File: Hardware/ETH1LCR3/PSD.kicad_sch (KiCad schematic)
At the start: 12 parts, among them U701 SN74LVC1G3157DB, U702 SN74LVC1G3157DB, U703 SN74LV1T34DBV, U704 SN74LV1T34DBV, U705 SN74LV1T34DBV, U706 TLV3501AIDBV

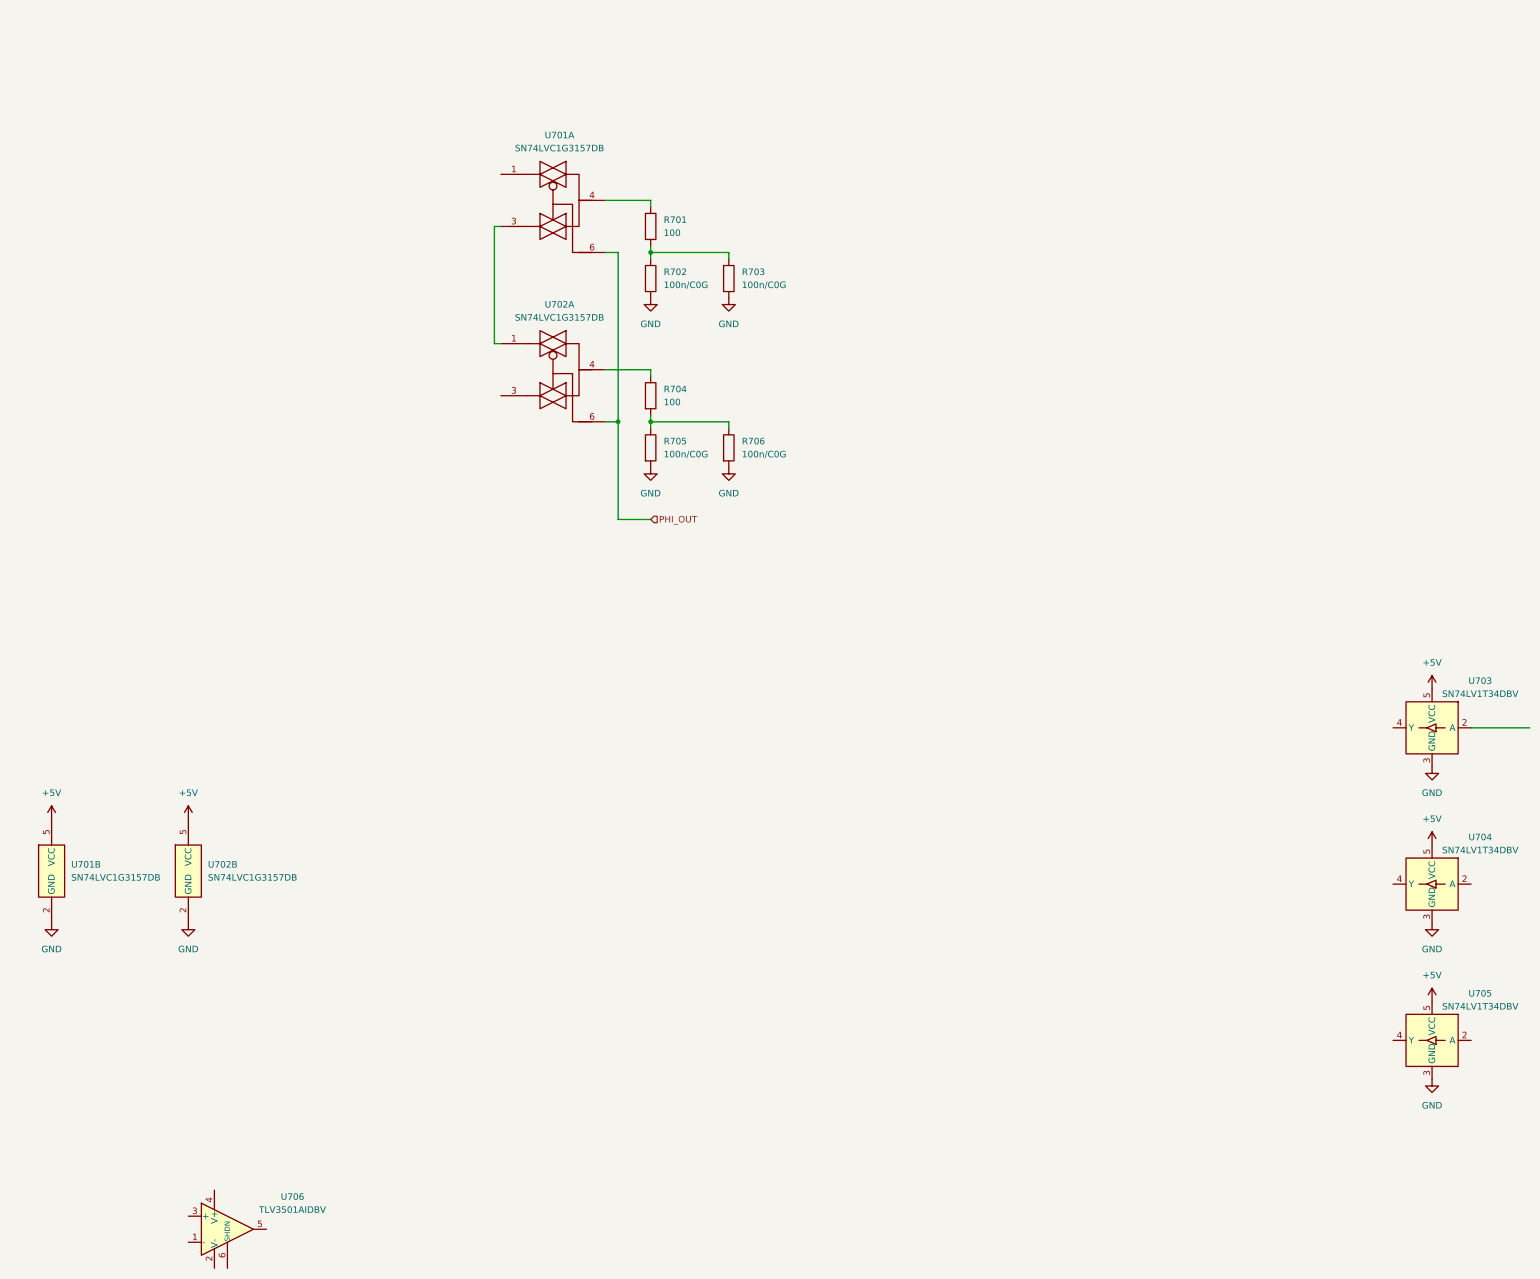
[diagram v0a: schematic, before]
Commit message: Hardware
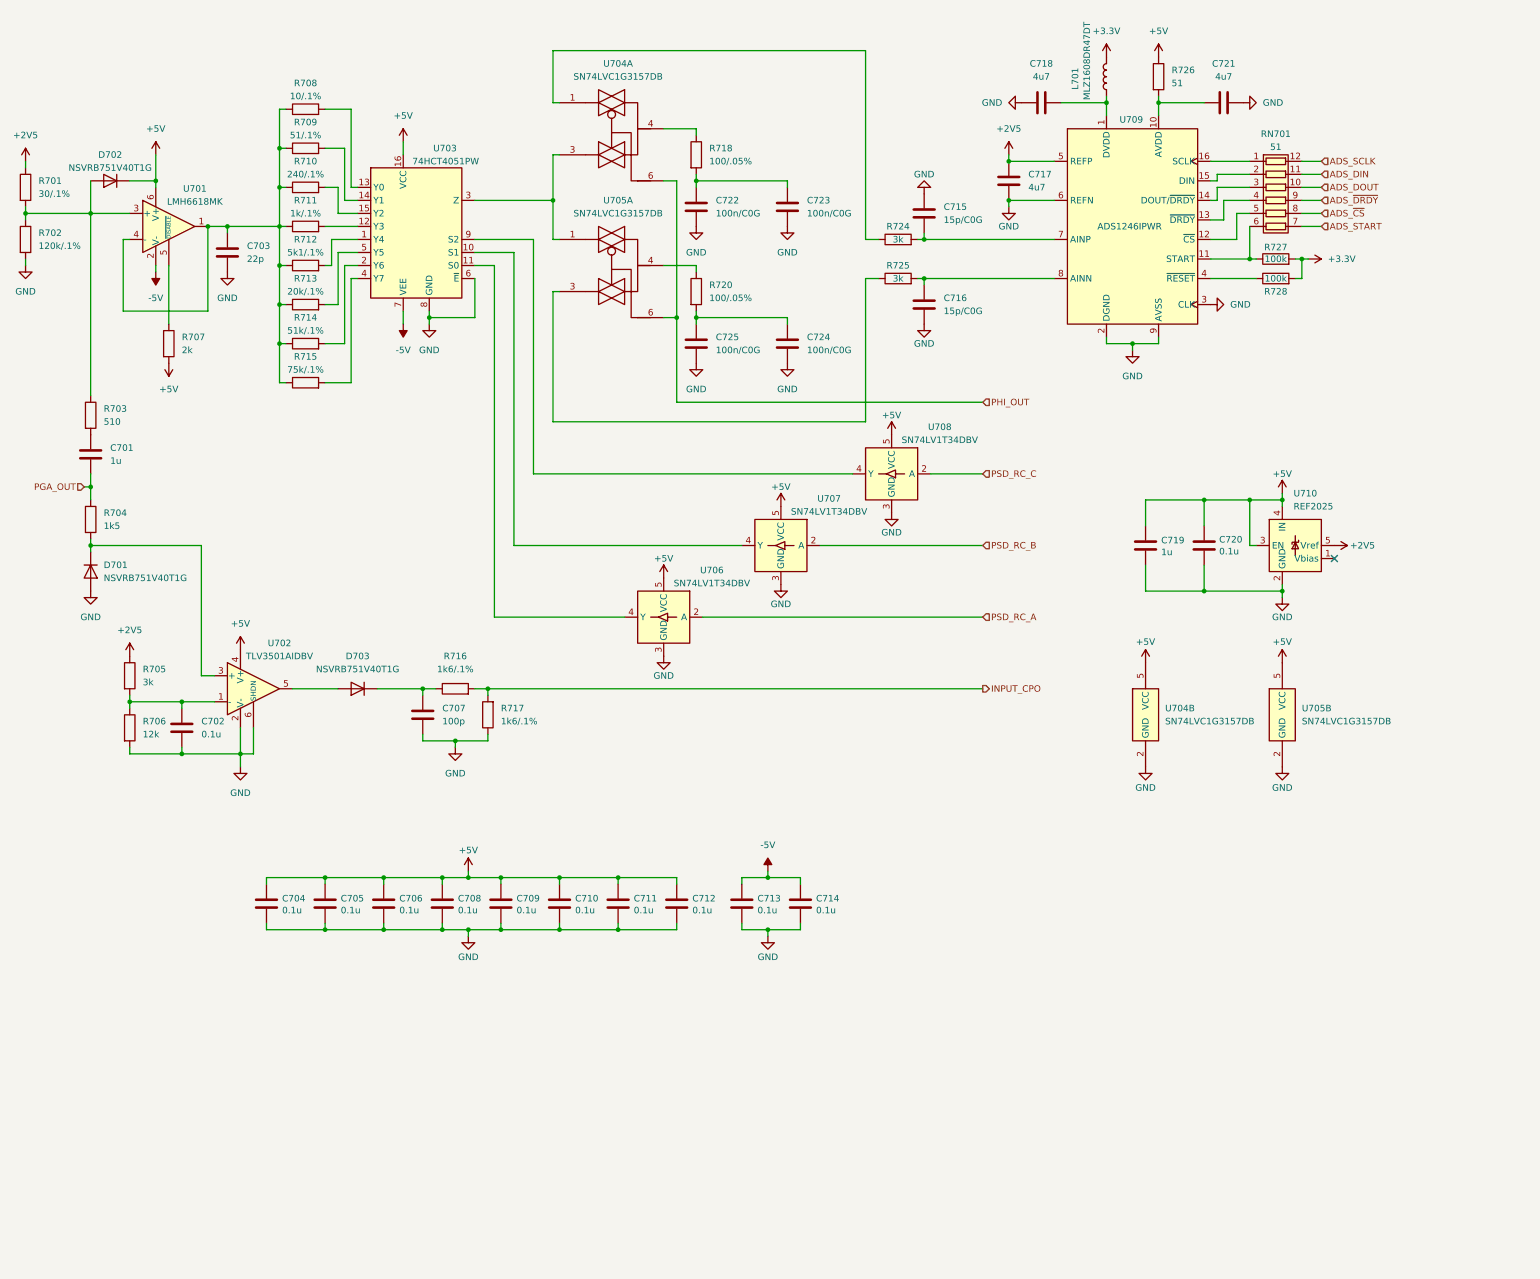
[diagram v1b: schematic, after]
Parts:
- added C701, C719: 1u, Capacitor_SMD:C_0603_1608Metric_Pad1.08x0.95mm_HandSolder, symbol Device:C
- added C702, C704, C705, C706, C708, C709, C710, C711, C712, C713, C714, C720: 0.1u, Capacitor_SMD:C_0603_1608Metric_Pad1.08x0.95mm_HandSolder, symbol Device:C
- added C703: 22p, Capacitor_SMD:C_0603_1608Metric_Pad1.08x0.95mm_HandSolder, symbol Device:C
- added C707: 100p, Capacitor_SMD:C_0603_1608Metric_Pad1.08x0.95mm_HandSolder, symbol Device:C
- added C715, C716: 15p/C0G, symbol Device:C
- added C717, C718, C721: 4u7, symbol Device:C
- added C722, C723, C724, C725: 100n/C0G, symbol Device:C
- added D701, D702, D703: NSVRB751V40T1G, symbol Device:D
- added L701: MLZ1608DR47DT, Inductor_SMD:L_0603_1608Metric_Pad1.05x0.95mm_HandSolder, symbol Device:L
- added R701: 30/.1%, Resistor_SMD:R_0603_1608Metric_Pad0.98x0.95mm_HandSolder, symbol Device:R
- added R704: 1k5, Resistor_SMD:R_0603_1608Metric_Pad0.98x0.95mm_HandSolder, symbol Device:R
- added R707: 2k, Resistor_SMD:R_0603_1608Metric_Pad0.98x0.95mm_HandSolder, symbol Device:R
- added R708: 10/.1%, Resistor_SMD:R_0603_1608Metric_Pad0.98x0.95mm_HandSolder, symbol Device:R
- added R709: 51/.1%, Resistor_SMD:R_0603_1608Metric_Pad0.98x0.95mm_HandSolder, symbol Device:R
- added R710: 240/.1%, Resistor_SMD:R_0603_1608Metric_Pad0.98x0.95mm_HandSolder, symbol Device:R
- added R711: 1k/.1%, Resistor_SMD:R_0603_1608Metric_Pad0.98x0.95mm_HandSolder, symbol Device:R
- added R712: 5k1/.1%, Resistor_SMD:R_0603_1608Metric_Pad0.98x0.95mm_HandSolder, symbol Device:R
- added R713: 20k/.1%, Resistor_SMD:R_0603_1608Metric_Pad0.98x0.95mm_HandSolder, symbol Device:R
- added R714: 51k/.1%, Resistor_SMD:R_0603_1608Metric_Pad0.98x0.95mm_HandSolder, symbol Device:R
- added R715: 75k/.1%, Resistor_SMD:R_0603_1608Metric_Pad0.98x0.95mm_HandSolder, symbol Device:R
- added R716, R717: 1k6/.1%, Resistor_SMD:R_0603_1608Metric_Pad0.98x0.95mm_HandSolder, symbol Device:R
- added R724, R725: 3k, Resistor_SMD:R_0603_1608Metric_Pad0.98x0.95mm_HandSolder, symbol Device:R
- added R726: 51, Resistor_SMD:R_0603_1608Metric_Pad0.98x0.95mm_HandSolder, symbol Device:R
- added R727, R728: 100k, Resistor_SMD:R_0603_1608Metric_Pad0.98x0.95mm_HandSolder, symbol Device:R
- added RN701: 51, symbol Device:R_Pack06
- added U701: LMH6618MK, Package_TO_SOT_SMD:TSOT-23-6_HandSoldering, symbol ETH1LCR3:LMH6618MK
- added U703: 74HCT4051PW, Package_SO:TSSOP-16_4.4x5mm_P0.65mm, symbol ETH1LCR3:74HCT4051PW
- added U709: ADS1246IPWR, Package_SO:TSSOP-16_4.4x5mm_P0.65mm, symbol ETH1LCR3:ADS1246IPWR
- added U710: REF2025, Package_TO_SOT_SMD:SOT-23-5, symbol Reference_Voltage:REF2025
- R702: value 100n/C0G -> 120k/.1%; footprint (none) -> Resistor_SMD:R_0603_1608Metric_Pad0.98x0.95mm_HandSolder
- R703: value 100n/C0G -> 510; footprint (none) -> Resistor_SMD:R_0603_1608Metric_Pad0.98x0.95mm_HandSolder
- R705: value 100n/C0G -> 3k; footprint (none) -> Resistor_SMD:R_0603_1608Metric_Pad0.98x0.95mm_HandSolder
- R706: value 100n/C0G -> 12k; footprint (none) -> Resistor_SMD:R_0603_1608Metric_Pad0.98x0.95mm_HandSolder
- R718: renamed from R701; value 100 -> 100/.05%; footprint (none) -> Resistor_SMD:R_0603_1608Metric_Pad0.98x0.95mm_HandSolder
- R720: renamed from R704; value 100 -> 100/.05%; footprint (none) -> Resistor_SMD:R_0603_1608Metric_Pad0.98x0.95mm_HandSolder
- U704: renamed from U701; footprint (none) -> Package_TO_SOT_SMD:SOT-23-6_Handsoldering
- U705: renamed from U702; footprint (none) -> Package_TO_SOT_SMD:SOT-23-6_Handsoldering
- renumbered U706 to U702, U705 to U706, U704 to U707, U703 to U708
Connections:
- net +5V: now also U702.4 (V+), C704.1, C705.1, C706.1, C708.1, C709.1, C710.1, C711.1, C712.1, C719.1, C720.1, D702.1 (K), R707.2, R726.1, U701.6 (V+), U703.16 (VCC), U710.3 (EN), U710.4 (IN)
- net GND: now also U702.2 (V-), U702.6 (SHDN), C702.2, C703.2, C704.2, C705.2, C706.2, C707.2, C708.2, C709.2, C710.2, C711.2, C712.2, C713.2, C714.2, C715.1, C716.2, C717.2, C718.1, C719.2, C720.2, C721.2, C722.2, C723.2, C724.2, C725.2, D701.2 (A), R717.1, U703.6 (~{E}), U703.8 (GND), U709.2 (DGND), U709.3 (CLK), U709.6 (REFN), U709.9 (AVSS), U710.2 (GND); no longer R703.2, R705.2
- net at U704.1: now also R724.1
- net at U704.3, U705.1: now also U703.3 (Z)
- net at R702.1, R703.1: now also D702.2 (A), R701.2, U701.3 (+); no longer R718.2
- net at U702.1 (-): now also R705.2, R706.1, C702.1
- net at U702.3 (+): now also D701.1 (K), R704.2
- net at U702.5: now also D703.2 (A)
- net PSD_RC_B: now reaches U707.2 (A)
- net at U707.4 (Y): now also U703.10 (S1)
- net PSD_RC_C: now reaches U708.2 (A)
- net at U708.4 (Y): now also U703.9 (S2)
- net at U705.3: now also R725.1
- net PSD_RC_A: now reaches U706.2 (A)
- net at U706.4 (Y): now also U703.11 (S0)
- new net: R707.1, U701.5 (~{DISABLE})
- new net: C703.1, R708.1, R709.1, R710.1, R711.1, R712.1, R713.1, R714.1, R715.1, U701.1, U701.4 (-)
- new net: R712.2, U703.1 (Y4)
- new net: C701.1, R703.2
- new net: R708.2, U703.13 (Y0)
- new net: C716.1, R725.2, U709.8 (AINN)
- new net: R713.2, U703.5 (Y5)
- new net: C722.1, C723.1, R718.2
- new net: C718.2, L701.1, U709.1 (DVDD)
- new net: R714.2, U703.2 (Y6)
- new net: C724.1, C725.1, R720.2
- new net: C721.1, R726.2, U709.10 (AVDD)
- new net: R710.2, U703.15 (Y2)
- new net: R711.2, U703.12 (Y3)
- new net: C715.2, R724.2, U709.7 (AINP)
- new net: R709.2, U703.14 (Y1)
- new net: R715.2, U703.4 (Y7)
- new net: R727.1, RN701.6 (R6.1), U709.11 (START)
- new net: RN701.5 (R5.1), U709.12 (~{CS})
- new net: RN701.4 (R4.1), U709.13 (~{DRDY})
- new net: RN701.3 (R3.1), U709.14 (DOUT/~{DRDY})
- new net: RN701.2 (R2.1), U709.15 (DIN)
- new net: RN701.1 (R1.1), U709.16 (SCLK)
- new net: R728.1, U709.4 (~{RESET})
- new net: C707.1, D703.1 (K), R716.1
- new net +2V5: C717.1, R701.1, R705.1, U709.5 (REFP), U710.5 (Vref)
- new net +3.3V: L701.2, R727.2, R728.2
- new net -5V: C713.1, C714.1, U701.2 (V-), U703.7 (VEE)
- new net ADS_DIN: RN701.11 (R2.2)
- new net ADS_DOUT: RN701.10 (R3.2)
- new net ADS_SCLK: RN701.12 (R1.2)
- new net ADS_START: RN701.7 (R6.2)
- new net ADS_~{CS}: RN701.8 (R5.2)
- new net ADS_~{DRDY}: RN701.9 (R4.2)
- new net INPUT_CPO: R716.2, R717.2
- new net PGA_OUT: C701.2, R704.1
- no-connect marks 0 -> 1
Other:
- moved on the sheet: R718, R720, U702, U704A, U704B, U705A, U705B, U706, U707, U708
